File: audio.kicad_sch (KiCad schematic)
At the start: 11 parts, among them J10 Audio IN Left, J11 Audio OUT Right, J12 Audio OUT Left, J6 USB_A, J7 Raspberry_pi, J8 HiFi Berry, J9 Audio IN Right

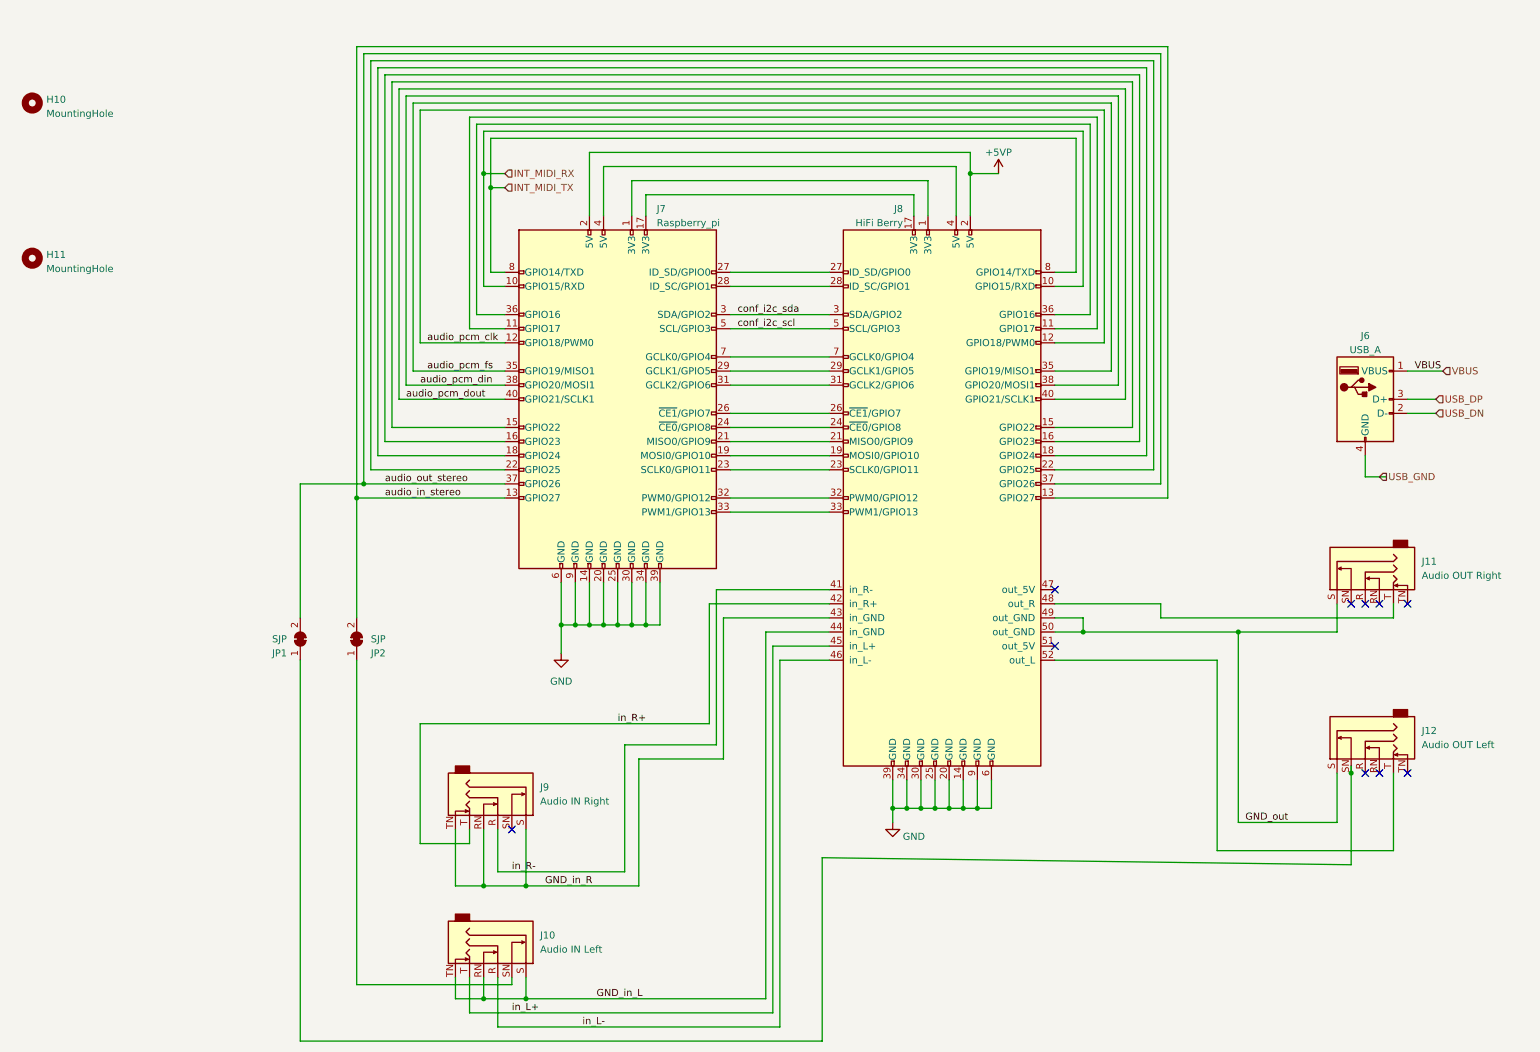
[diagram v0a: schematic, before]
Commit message: Initial Revision of CM4
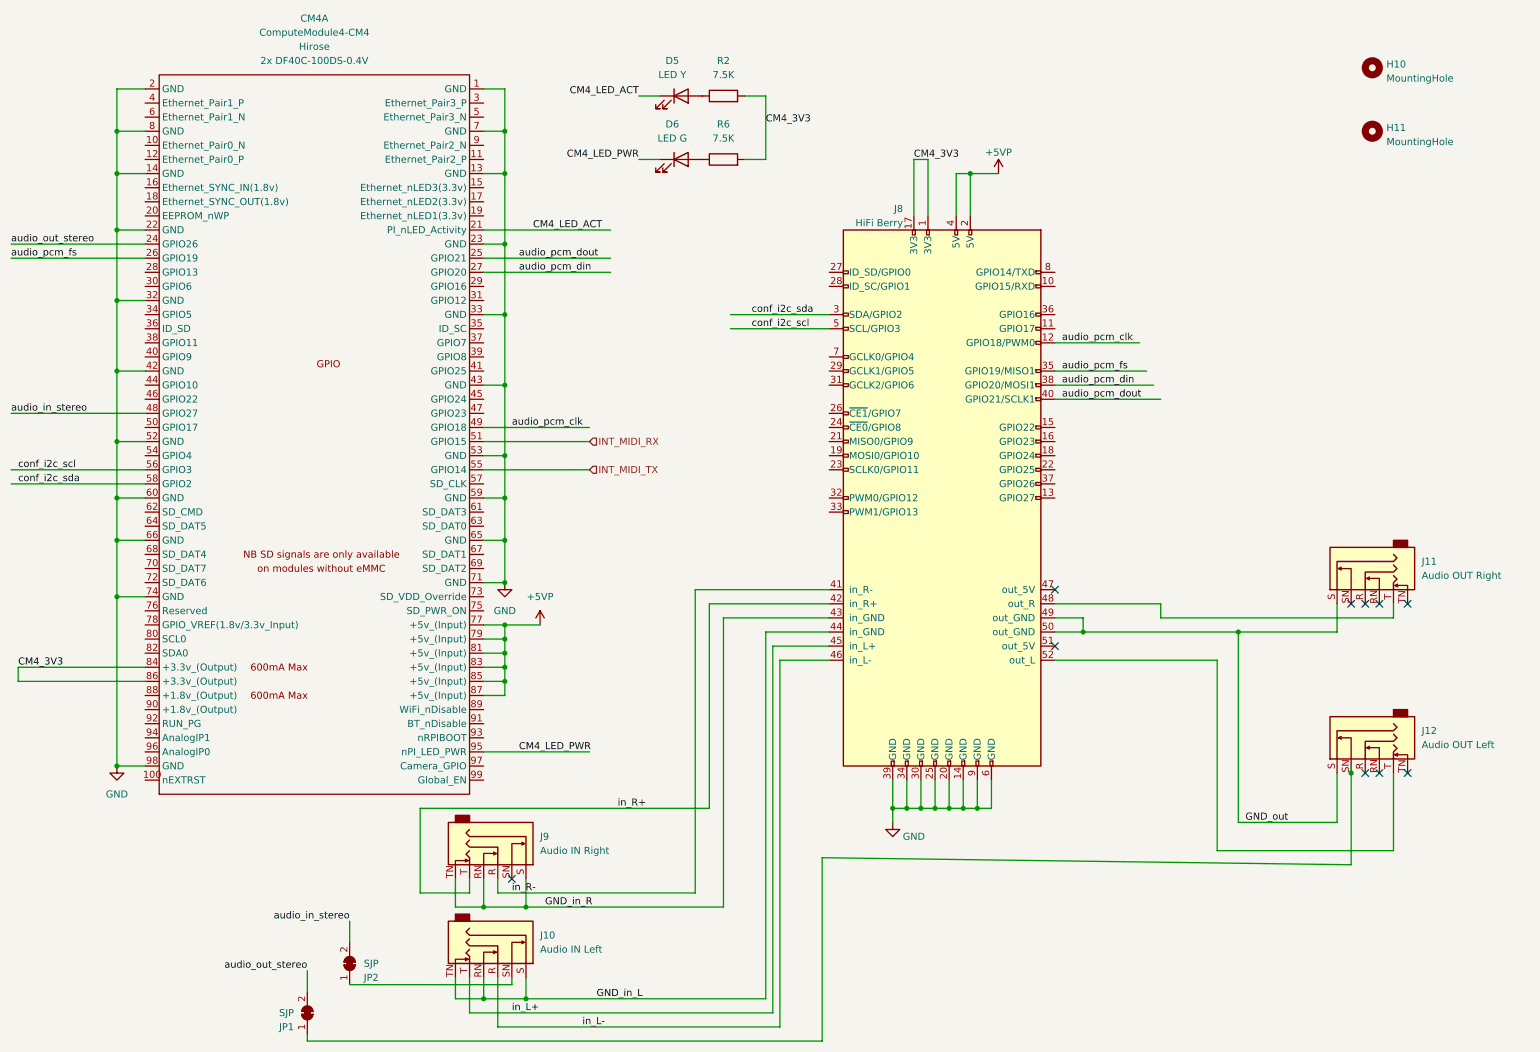
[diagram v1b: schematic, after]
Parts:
- removed J6: USB_A, Pedalboard Library:USB A BCB Male Plug, symbol Connector:USB_A
- removed J7: Raspberry_pi, Pedalboard Library:Raspberry PI Compute Module CM4 Nano A, symbol Connector:Raspberry_Pi_2_3
- added CM4: ComputeModule4-CM4, Pedalboard Library:Raspberry-Pi-4-Compute-Module, symbol pedalboard:ComputeModule4-CM4
- added D5: LED Y, LED_SMD:LED_0805_2012Metric, symbol Device:LED
- added D6: LED G, LED_SMD:LED_0805_2012Metric, symbol Device:LED
- added R2, R6: 7.5K, Resistor_SMD:R_0805_2012Metric, symbol Device:R
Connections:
- net +5VP: now also J8.4 (5V), CM4.77 (+5v_(Input)), CM4.79 (+5v_(Input)), CM4.81 (+5v_(Input)), CM4.83 (+5v_(Input)), CM4.85 (+5v_(Input)), CM4.87 (+5v_(Input))
- net GND: now also CM4.1 (GND), CM4.13 (GND), CM4.14 (GND), CM4.2 (GND), CM4.22 (GND), CM4.23 (GND), CM4.32 (GND), CM4.33 (GND), CM4.42 (GND), CM4.43 (GND), CM4.52 (GND), CM4.53 (GND), CM4.59 (GND), CM4.60 (GND), CM4.65 (GND), CM4.66 (GND), CM4.7 (GND), CM4.71 (GND), CM4.74 (GND), CM4.8 (GND), CM4.98 (GND)
- net INT_MIDI_RX: now also CM4.51 (GPIO15); no longer J8.10 (GPIO15/RXD)
- net INT_MIDI_TX: now also CM4.55 (GPIO14); no longer J8.8 (GPIO14/TXD)
- net audio_in_stereo: now also CM4.48 (GPIO27); no longer J8.13 (GPIO27)
- net audio_out_stereo: now also CM4.24 (GPIO26); no longer J8.37 (GPIO26)
- net audio_pcm_clk: now also CM4.49 (GPIO18)
- net audio_pcm_din: now also CM4.27 (GPIO20)
- net audio_pcm_dout: now also CM4.25 (GPIO21)
- net audio_pcm_fs: now also CM4.26 (GPIO19)
- net conf_i2c_scl: now also CM4.56 (GPIO3)
- net conf_i2c_sda: now also CM4.58 (GPIO2)
- net CM4_3V3: now reaches J8.1 (3V3)
- net CM4_3V3: now also J8.17 (3V3), CM4.84 (+3.3v_(Output)), CM4.86 (+3.3v_(Output)), R2.2, R6.2
- new net: D5.2 (A), R2.1
- new net: D6.2 (A), R6.1
- new net CM4_LED_ACT: CM4.21 (PI_nLED_Activity), D5.1 (K)
- new net CM4_LED_PWR: CM4.95 (nPI_LED_PWR), D6.1 (K)
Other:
- moved on the sheet: H10, H11, J9, JP1, JP2
